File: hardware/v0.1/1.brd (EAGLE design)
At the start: 113 x 46.5 mm, 86 parts, among them IC1 FP6291, IC2 TM1809, IC3 STM32F10XCXT6, IC5 TSOP34830, IC6 TSOP34830, Q1 8050, Q2 8050, U1 74LVC1G08SE-7, Y1 8M

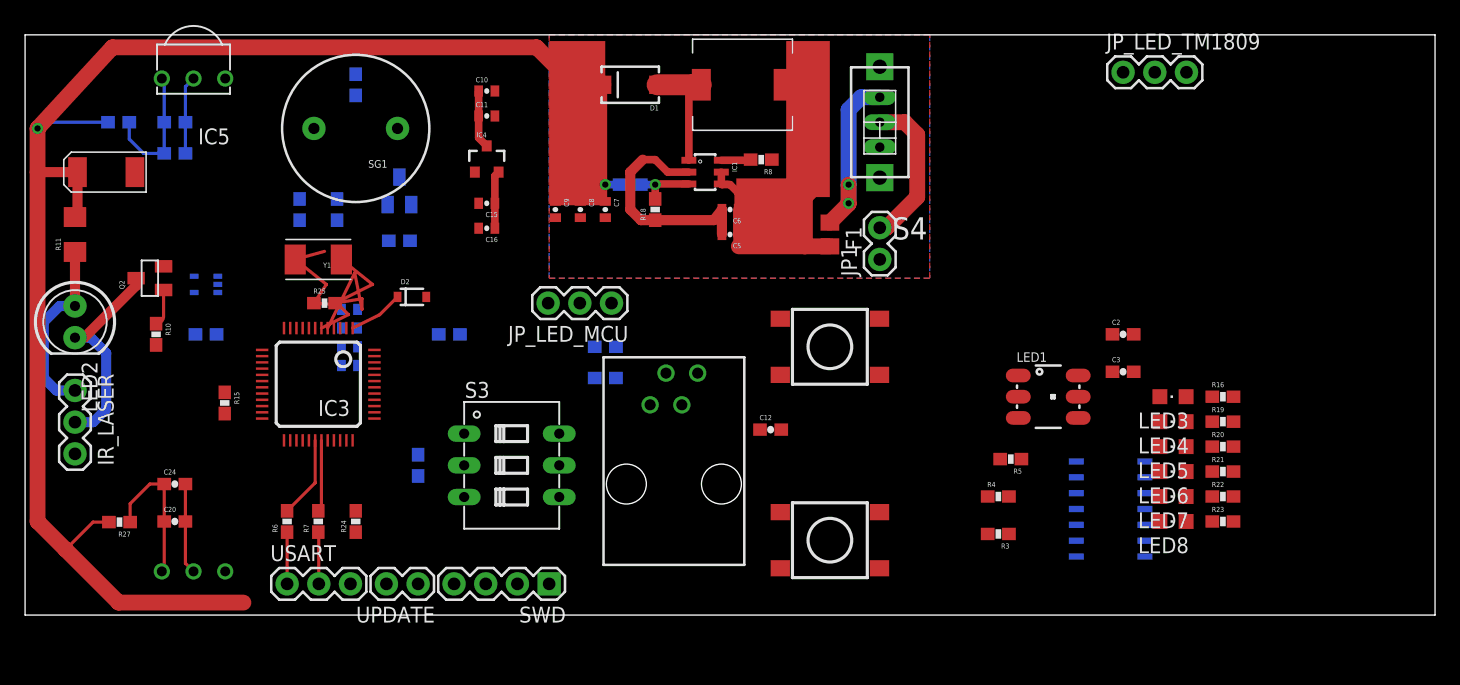
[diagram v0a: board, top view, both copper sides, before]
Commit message: nearly finish
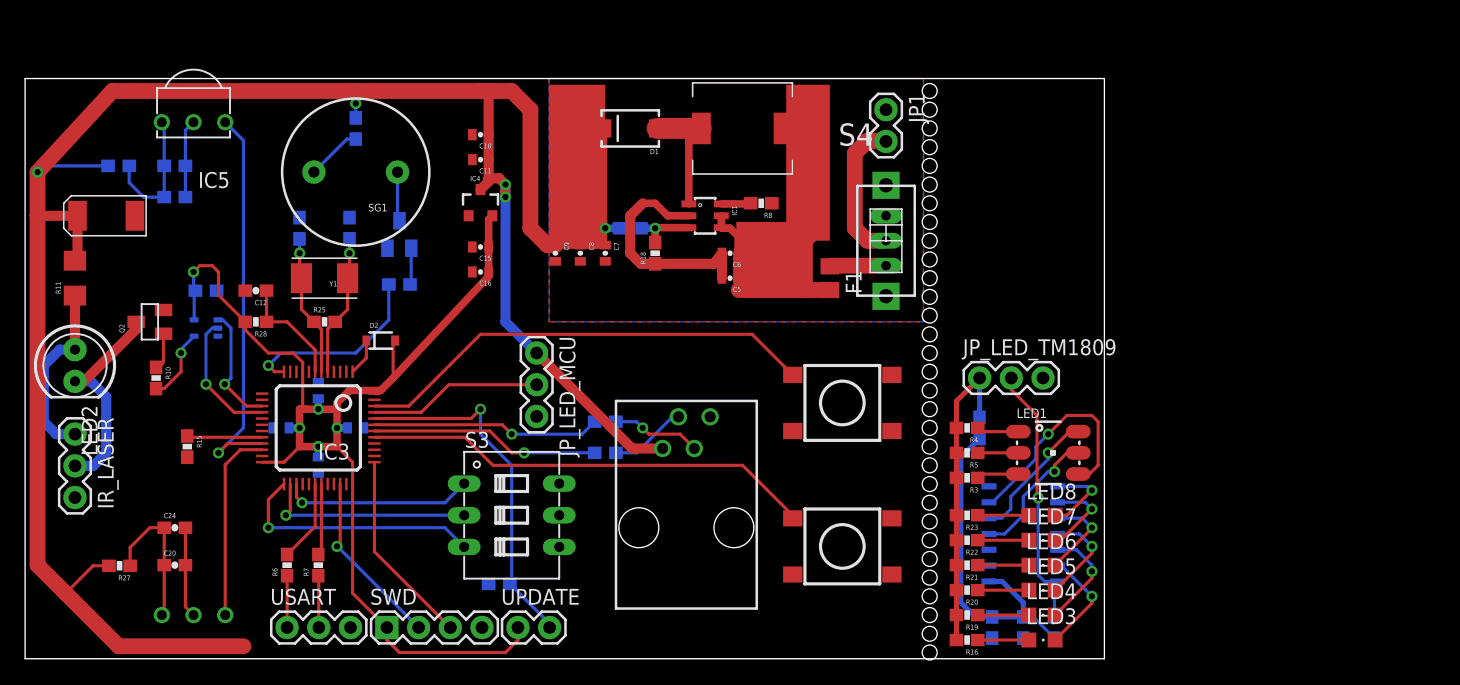
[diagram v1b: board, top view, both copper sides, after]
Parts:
- added R28: 10K, SparkFun-Passives:0603-RES
- moved R12 53.9 mm to (82.5, 2.50), turned to 270 degrees
- moved R9 45.1 mm to (76.5, 18.5), turned to 90 degrees
- moved C12 42.7 mm to (18.5, 29.5), turned to 180 degrees
- moved R16 28.3 mm to (75.5, 1.50), turned to 180 degrees
- moved JP_LED_TM1809 27.1 mm to (76.5, 22.5)
- moved C2 25.7 mm to (77.5, 2.50), flipped to the bottom, turned to 90 degrees
- moved R19 25.7 mm to (75.5, 3.50), turned to 180 degrees
- moved R20 23.5 mm to (75.5, 5.50), turned to 180 degrees
- moved LED3 22.1 mm to (81.5, 1.50), turned to 270 degrees
- moved C3 22.0 mm to (80.0, 2.50), flipped to the bottom, turned to 90 degrees
- moved R21 21.8 mm to (75.5, 7.50), turned to 180 degrees
- moved R22 20.8 mm to (75.5, 9.50), turned to 180 degrees
- moved R23 20.5 mm to (75.5, 11.5), turned to 180 degrees
- moved LED4 18.7 mm to (81.5, 3.50), turned to 270 degrees
- moved LED5 15.6 mm to (81.5, 5.50), turned to 270 degrees
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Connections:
- new net N$44: C12.1, IC3.7, R28.1
- net 3.3V: now also R28.2; no longer C12.1, IC3.7
- net 5V: no longer C2.1, C3.1, R12.2
- net BTN_RELOAD: now also IC3.46
- net BTN_TRIGGER: now also IC3.41
- net BUZZER: now also IC3.12
- net DIP_SW1: now also IC3.27
- net DIP_SW2: now also IC3.26
- net DIP_SW3: now also IC3.25
- net GND: now also C2.1, C3.1, JP_LED_MCU.3, JP_LED_TM1809.3; no longer C2.2, C3.2, JP_LED_MCU.2, JP_LED_TM1809.2
- net IR_EMITTER: now also IC3.15
- net IR_RECEIVE1: now also IC3.21
- net IR_RECEIVE2: now also IC3.22
- net LED_MCU: now also IC3.45, JP_LED_MCU.2; no longer JP_LED_MCU.3
- net LED_TM: now also JP_LED_TM1809.2; no longer JP_LED_TM1809.3
- net N$36: now also C2.2, C3.2, R12.2
- net PWM_38K: now also IC3.16
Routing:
- net 3.3V: track 4.62 -> 95.8 mm, vias 0 -> 5
- net 5V: track 136.9 -> 203.8 mm, vias 2 -> 5
- net BTN_RELOAD: track 0.00 -> 37.3 mm
- net BTN_TRIGGER: track 0.00 -> 36.3 mm
- net IR_RECEIVE1: track 0.00 -> 31.7 mm, vias 0 -> 1
- net N$2: track 0.00 -> 28.7 mm, vias 0 -> 1
- net N$36: track 0.00 -> 27.1 mm
- net LED_TM: track 0.00 -> 21.4 mm, vias 0 -> 1
- net DIP_SW3: track 0.00 -> 20.3 mm, vias 0 -> 1
- net N$39: track 0.00 -> 20.2 mm, vias 0 -> 1
- net N$40: track 0.00 -> 18.4 mm, vias 0 -> 1
- net N$16: track 0.00 -> 17.8 mm, vias 0 -> 1
- net DIP_SW2: track 0.00 -> 16.9 mm, vias 0 -> 1
- net SWDCLK: track 0.00 -> 15.8 mm
- net IR_RECEIVE2: track 0.00 -> 15.5 mm
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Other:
- board size 113 x 46.5 mm -> 86.5 x 46.5 mm

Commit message: finish wire
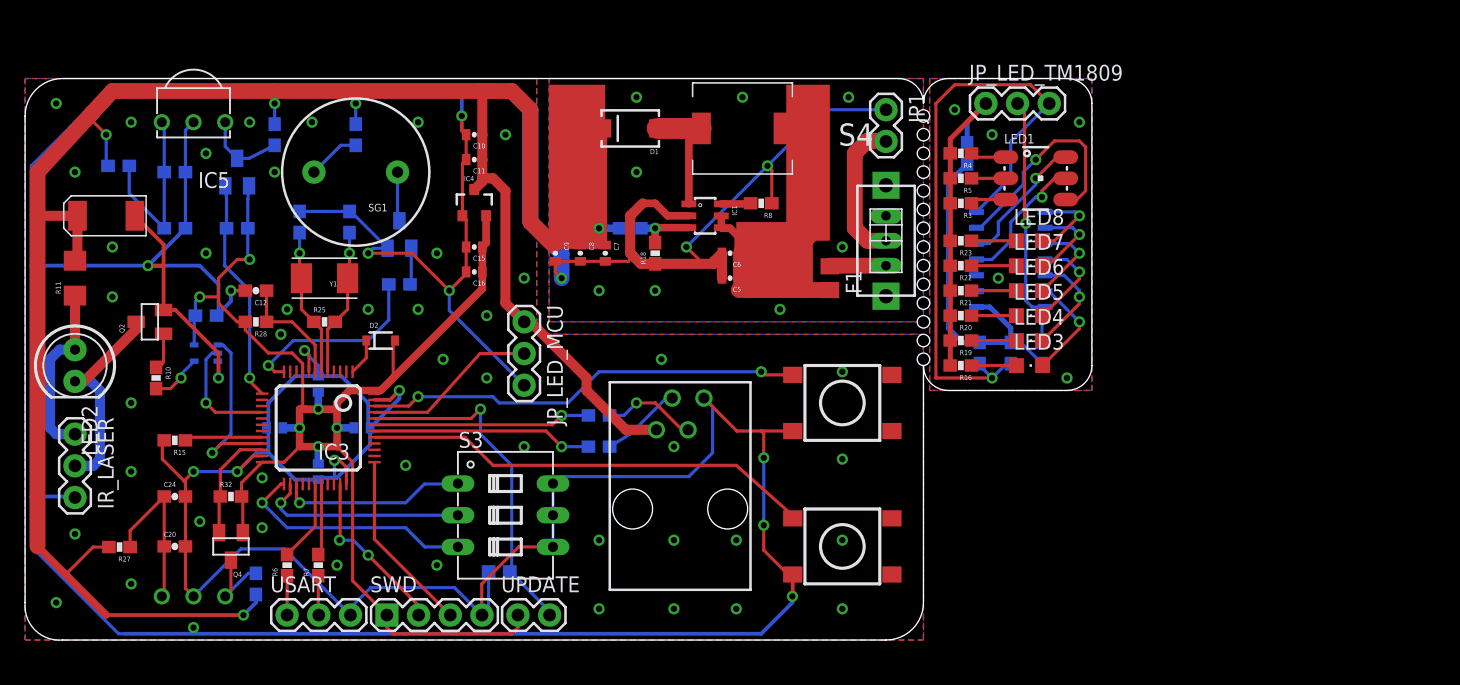
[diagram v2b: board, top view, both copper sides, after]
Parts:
- added Q3, Q4: 2N7002, SparkFun-DiscreteSemi:SOT23
- added R29, R30: 47K, SparkFun-Passives:0603-RES
- added R31, R32: 10K, SparkFun-Passives:0603-RES
- R13, R14: value 220R -> 100R
- R17: value 110K -> 110K(47K)
- R18: value 15K -> 15K(6.4K)
- moved C2 22.0 mm to (76.5, 24.5)
- moved C3 22.0 mm to (79.0, 24.5)
- moved IC2 22.0 mm to (79.0, 32.0)
- moved LED1 22.0 mm to (81.0, 38.5)
- moved LED3 22.0 mm to (80.5, 23.5)
- moved LED4 22.0 mm to (80.5, 25.5)
- moved LED5 22.0 mm to (80.5, 27.5)
- moved LED6 22.0 mm to (80.5, 29.5)
- moved LED7 22.0 mm to (80.5, 31.5)
- moved LED8 22.0 mm to (80.5, 33.5)
- moved R12 22.0 mm to (81.5, 24.5)
- moved R9 22.0 mm to (75.5, 40.5)
- moved JP_LED_TM1809 22.0 mm to (77.0, 44.5)
- moved R16 22.0 mm to (75.0, 23.5)
- moved R19 22.0 mm to (75.0, 25.5)
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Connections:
- new net N$45: IC5.1, Q3.3, R30.1
- new net N$47: IC6.1, Q4.3, R29.1
- net 3.3V: now also Q3.1, Q4.1, R31.2, R32.2
- net 5V: now also R29.2, R30.2
- net IR_EMITTER: now also IC3.21; no longer IC3.15
- net IR_RECEIVE1: now also IC3.13, Q3.2, R31.1; no longer IC3.21, IC5.1
- net IR_RECEIVE2: now also Q4.2, R32.1; no longer IC6.1
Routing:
- net GND: track 32.2 -> 514.7 mm, vias 0 -> 76
- net 3.3V: track 95.8 -> 110.8 mm, vias 5 -> 6
- net IR_RECEIVE1: track 31.7 -> 18.0 mm
- net N$45: track 0.00 -> 6.55 mm
- net IR_RECEIVE2: track 15.5 -> 9.10 mm
- net N$47: track 0.00 -> 6.32 mm
- net IR_EMITTER: track 9.75 -> 14.3 mm
- net N$11: track 10.7 -> 14.7 mm
- net N$39: track 20.2 -> 17.5 mm
- net BTN_RELOAD: track 37.3 -> 35.2 mm, vias 0 -> 2
- net N$6: track 5.84 -> 4.14 mm
- net 5V: track 203.8 -> 205.4 mm
- net N$12: track 11.9 -> 13.3 mm
- net PWM_38K: track 10.6 -> 9.47 mm
- net USART_TX: track 4.15 -> 3.15 mm
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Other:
- board size 86.5 x 46.5 mm -> 85.5 x 45 mm
